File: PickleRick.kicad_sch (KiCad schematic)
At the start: 56 parts, among them J1 RBUS, J12 Conn_01x03_Male, J2 Conn_01x02_Male, J3 292227-7, J4 Micro_SD_Card_Det, Q1 PMV20ENR, U1 ESP32-S3, U2 DPS310, Y1 40MHz±10ppm

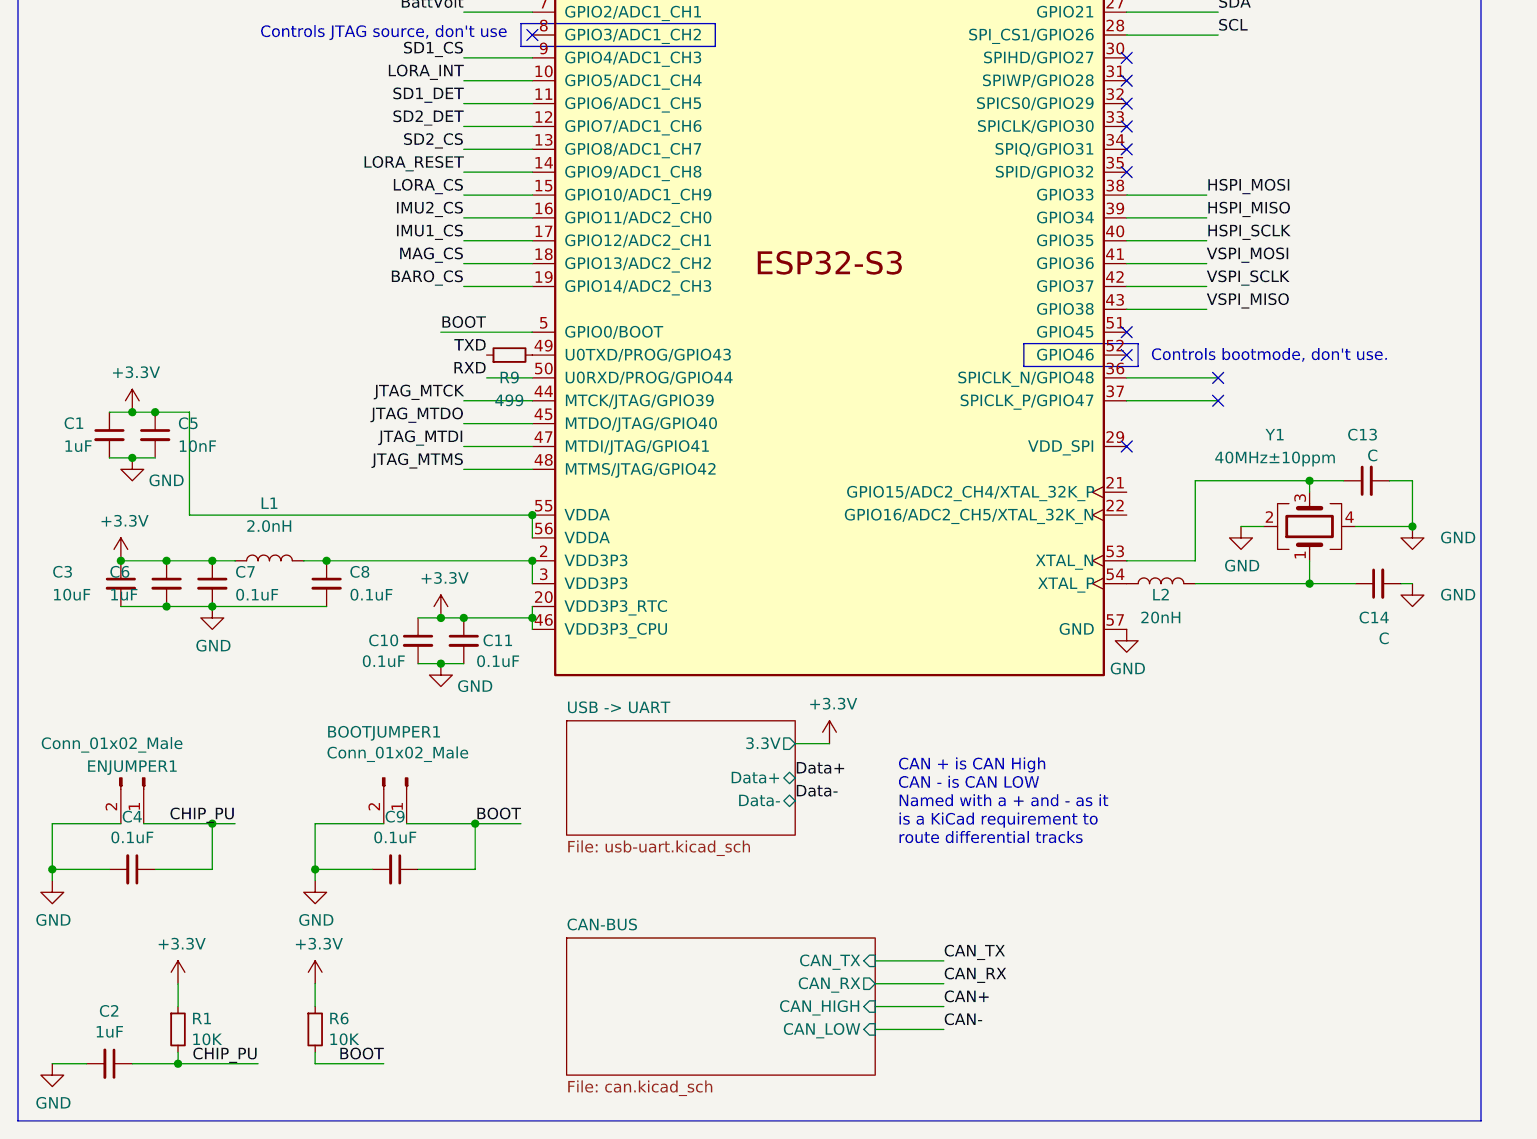
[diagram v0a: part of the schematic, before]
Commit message: layout almost complete
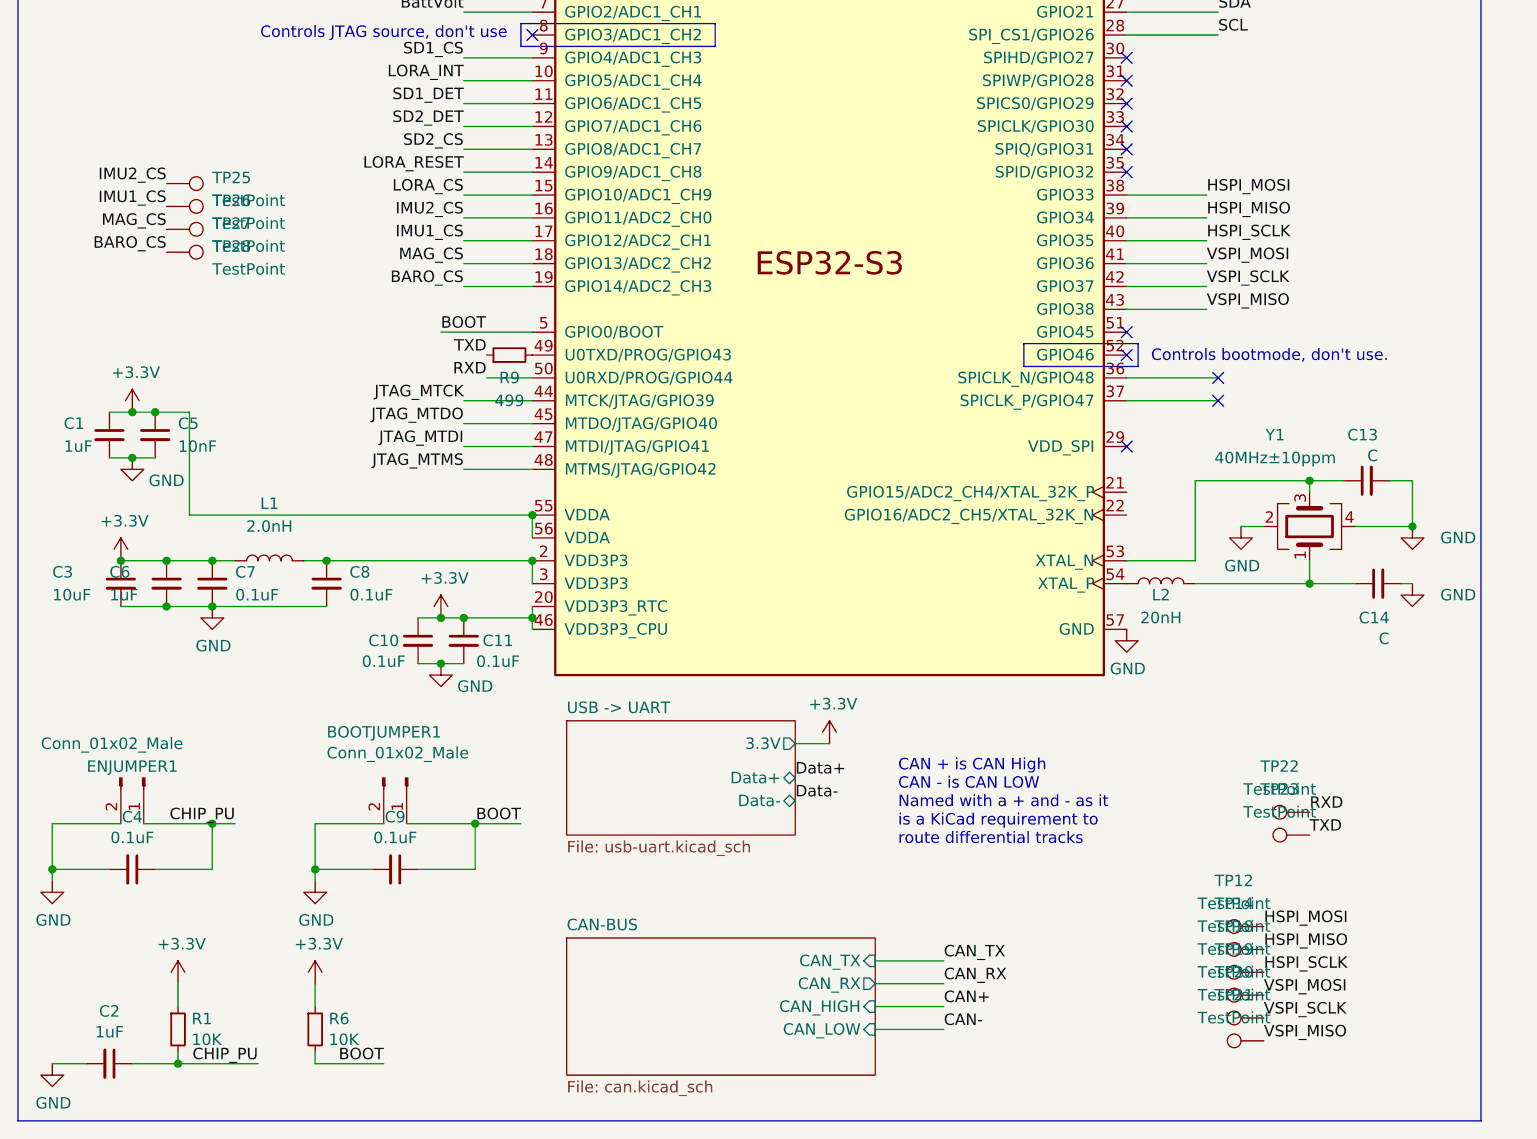
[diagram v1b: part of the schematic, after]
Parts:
- added TP12, TP14, TP18, TP19, TP20, TP21, TP22, TP23, TP25, TP26, TP27, TP28: TestPoint, TestPoint:TestPoint_Pad_D1.0mm, symbol Connector:TestPoint
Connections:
- net BARO_CS: now also TP28.1
- net HSPI_MISO: now also TP14.1
- net HSPI_MOSI: now also TP12.1
- net HSPI_SCLK: now also TP18.1
- net IMU1_CS: now also TP26.1
- net IMU2_CS: now also TP25.1
- net MAG_CS: now also TP27.1
- net RXD: now also TP22.1
- net TXD: now also TP23.1
- net VSPI_MISO: now also TP21.1
- net VSPI_MOSI: now also TP19.1
- net VSPI_SCLK: now also TP20.1
